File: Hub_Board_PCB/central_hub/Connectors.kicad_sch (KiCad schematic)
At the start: 15 parts, among them J3 Screw_Terminal_01x08, J4 Screw_Terminal_01x08, J5 CSP-USC16-TR, J6 Screw_Terminal_01x04, J6 Screw_Terminal_01x06, J7 Conn_01x03, J8 Conn_01x02

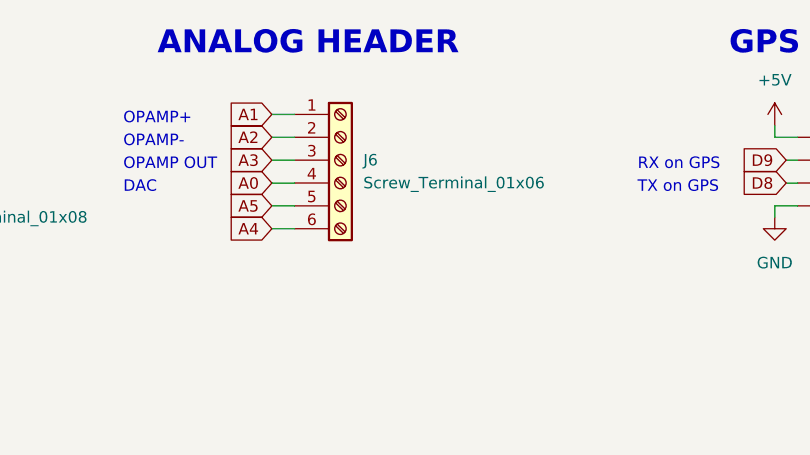
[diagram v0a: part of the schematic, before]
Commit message: Schematic changes before sending to kim
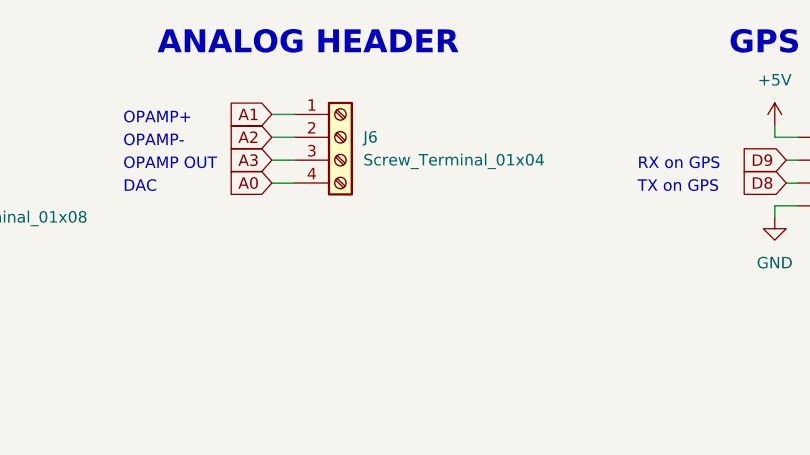
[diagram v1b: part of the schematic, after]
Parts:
- removed J6: Screw_Terminal_01x06, Connector_PinHeader_2.54mm:PinHeader_1x06_P2.54mm_Vertical, symbol Connector:Screw_Terminal_01x06
- added J6: Screw_Terminal_01x04, Connector_PinHeader_2.54mm:PinHeader_1x04_P2.54mm_Vertical, symbol Connector:Screw_Terminal_01x04
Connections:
- net A0: now also J6.4
- net A1: now also J6.1
- net A2: now also J6.2
- net A3: now also J6.3
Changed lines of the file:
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@@
-    (stroke (width 0) (type default))
-  )
-  (wire (pts (xy 92.71 43.18) (xy 95.25 43.18))
     (stroke (width 0) (type default))
   )
@@
   )
   (wire (pts (xy 43.18 49.53) (xy 44.45 49.53))
-    (stroke (width 0) (type default))
-  )
-  (wire (pts (xy 92.71 40.64) (xy 95.25 40.64))
     (stroke (width 0) (type default))
   )
@@
     (effects (font (size 1.27 1.27)) (justify right))
     (property "Intersheetrefs" "${INTERSHEET_REFS}" (at 87.4267 33.02 0)
-      (effects (font (size 1.27 1.27)) (justify right) hide)
-    )
-  )
-  (global_label "A5" (shape input) (at 92.71 40.64 180) (fields_autoplaced)
-    (effects (font (size 1.27 1.27)) (justify right))
-    (property "Intersheetrefs" "${INTERSHEET_REFS}" (at 87.4267 40.64 0)
       (effects (font (size 1.27 1.27)) (justify right) hide)
     )
@@
     (effects (font (size 1.27 1.27)) (justify right))
     (property "Intersheetrefs" "${INTERSHEET_REFS}" (at 87.4267 38.1 0)
-      (effects (font (size 1.27 1.27)) (justify right) hide)
-    )
-  )
-  (global_label "A4" (shape input) (at 92.71 43.18 180) (fields_autoplaced)
-    (effects (font (size 1.27 1.27)) (justify right))
-    (property "Intersheetrefs" "${INTERSHEET_REFS}" (at 87.4267 43.18 0)
       (effects (font (size 1.27 1.27)) (justify right) hide)
     )
@@
         (path "/4ad82a24-c992-45c9-b523-12e12bcd6ced/996060af-581e-425f-9e10-26ee39d5a960"
           (reference "J8") (unit 1)
+        )
+      )
+    )
+  )
+  (symbol (lib_id "Connector:Screw_Terminal_01x04") (at 100.33 33.02 0) (unit 1)
+    (in_bom yes) (on_board yes) (dnp no) (fields_autoplaced)
+    (property "Reference" "J6" (at 102.87 33.02 0)
+      (effects (font (size 1.27 1.27)) (justify left))
+    )
+    (property "Value" "Screw_Terminal_01x04" (at 102.87 35.56 0)
+      (effects (font (size 1.27 1.27)) (justify left))
+    )
+    (property "Footprint" "Connector_PinHeader_2.54mm:PinHeader_1x04_P2.54mm_Vertical" (at 100.33 33.02 0)
+      (effects (font (size 1.27 1.27)) hide)
+    )
+    (property "Datasheet" "~" (at 100.33 33.02 0)
+      (effects (font (size 1.27 1.27)) hide)
+    )
+    (pin "1")
+    (pin "2")
+    (pin "3")
+    (pin "4")
+    (instances
+      (project "central_hub"
+        (path "/0d9ec66e-0fbf-4d12-9b83-adf78971a00b"
+          (reference "J6") (unit 1)
+        )
+        (path "/0d9ec66e-0fbf-4d12-9b83-adf78971a00b/4fb60496-ee10-4e45-a75e-a49c2c8afc68"
+          (reference "J14") (unit 1)
+        )
+        (path "/0d9ec66e-0fbf-4d12-9b83-adf78971a00b/8e53aed1-21e6-440d-aae4-1b5509ec346a"
+          (reference "J6") (unit 1)
         )
       )
@@
         )
       )
-    )
-  )
-  (symbol (lib_id "Connector:Screw_Terminal_01x06") (at 100.33 35.56 0) (unit 1)
-    (in_bom yes) (on_board yes) (dnp no) (fields_autoplaced)
-    (property "Reference" "J6" (at 102.87 35.56 0)
-      (effects (font (size 1.27 1.27)) (justify left))
-    )
-    (property "Value" "Screw_Terminal_01x06" (at 102.87 38.1 0)
-      (effects (font (size 1.27 1.27)) (justify left))
-    )
-    (property "Footprint" "Connector_PinHeader_2.54mm:PinHeader_1x06_P2.54mm_Vertical" (at 100.33 35.56 0)
-      (effects (font (size 1.27 1.27)) hide)
-    )
-    (property "Datasheet" "~" (at 100.33 35.56 0)
-      (effects (font (size 1.27 1.27)) hide)
-    )
-    (pin "1")
-    (pin "2")
-    (pin "3")
-    (pin "4")
-    (pin "5")
-    (pin "6")
-    (instances
-      (project "central_hub"
-        (path "/0d9ec66e-0fbf-4d12-9b83-adf78971a00b/8e53aed1-21e6-440d-aae4-1b5509ec346a"
-          (reference "J6") (unit 1)
-        )
-      )
